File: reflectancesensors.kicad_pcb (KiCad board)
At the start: 2 copper layers, 71.5 x 47 mm, 22 parts, among them J1 Power, J2 Outputs, Q1 BPW40, Q2 BPW40, U1 TCRT5000L, U3 TCRT5000L

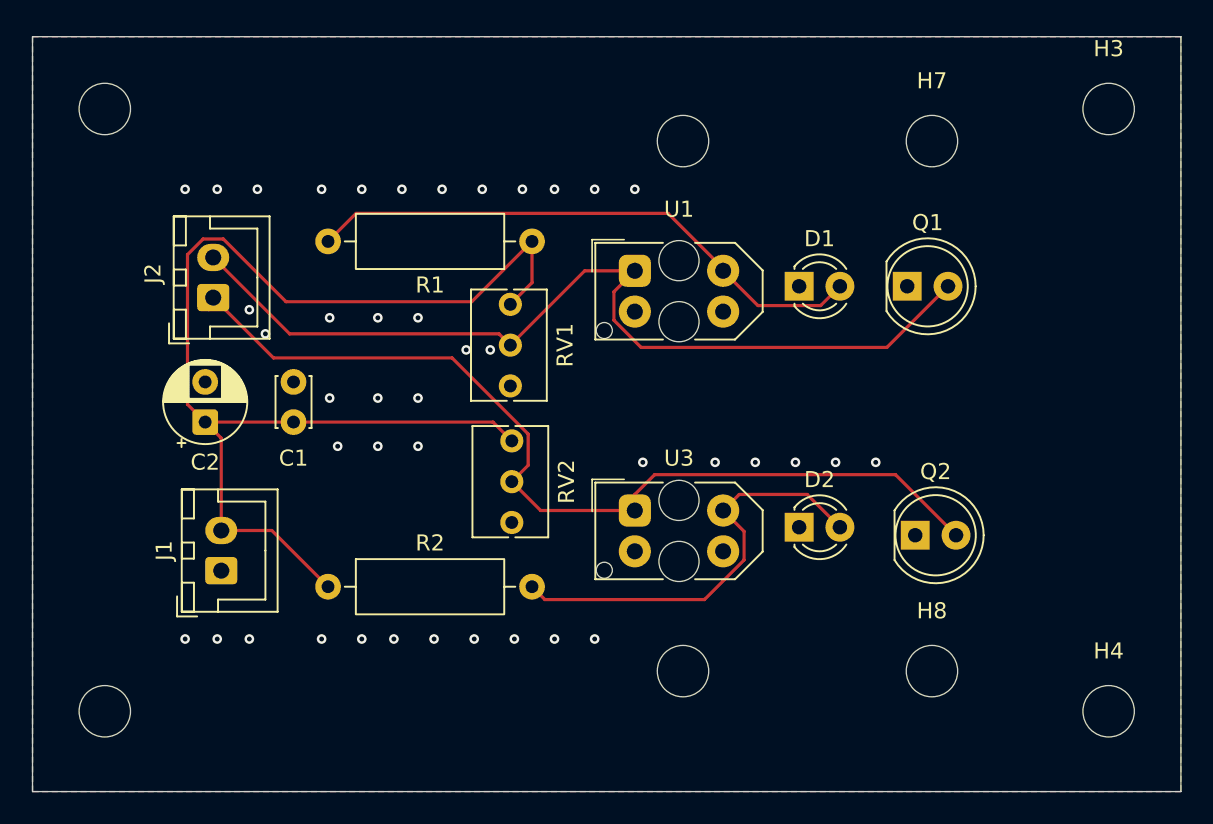
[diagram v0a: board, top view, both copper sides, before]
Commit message: small changes
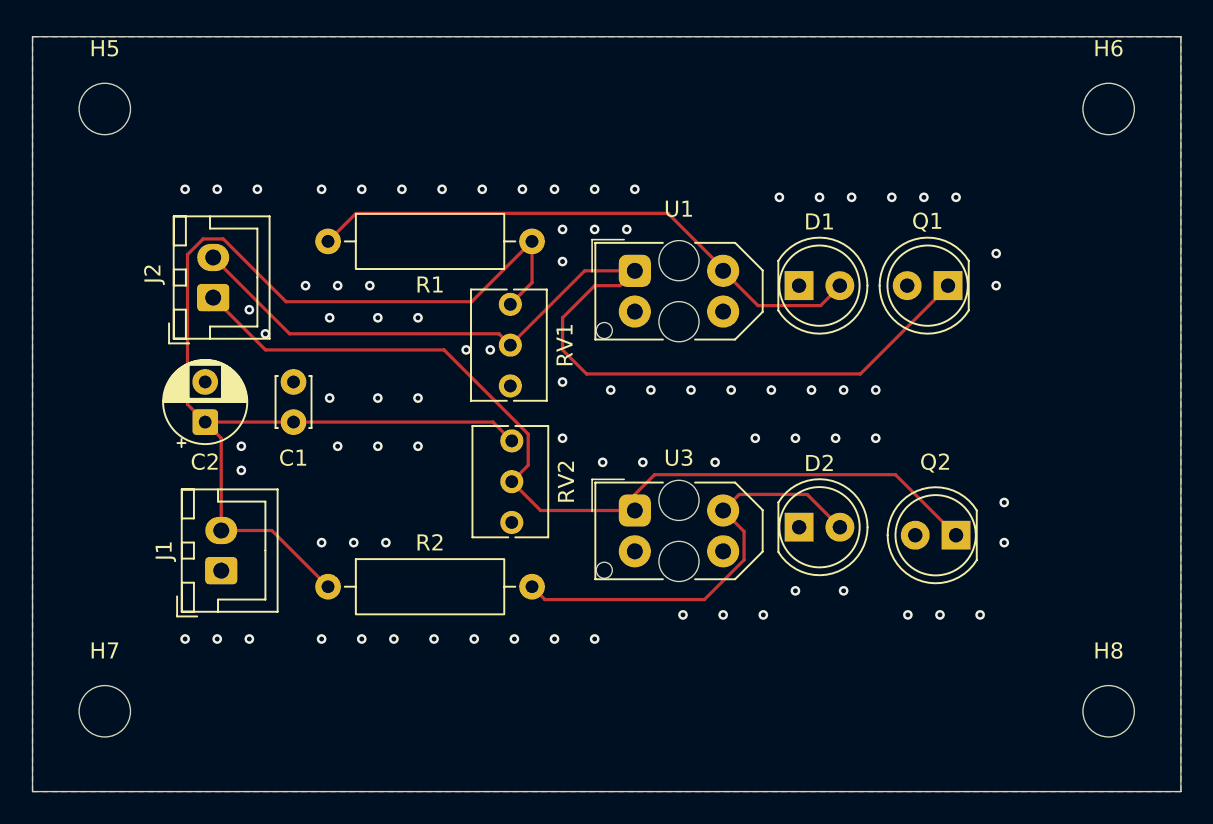
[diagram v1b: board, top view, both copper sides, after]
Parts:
- removed H1, H2, H3, H4: MountingHole, MountingHole:MountingHole_3.2mm_M3_DIN965
- D1, D2: footprint LED_THT:LED_D3.0mm_IRBlack -> LED_THT:LED_D5.0mm
- moved H7 62.5 mm to (82.5, 124.5)
- moved H6 43.9 mm to (145.0, 87.0)
- moved H5 36.1 mm to (82.5, 87.0)
- moved H8 11.3 mm to (145.0, 124.5)
- moved Q1 2.54 mm to (135.0, 98.0), turned to 180 degrees
- moved Q2 2.54 mm to (135.5, 113.5), turned to 180 degrees
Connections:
- Q1 pad 1: GND -> Net-(J2-Pin_2)
- Q1 pad 2: Net-(J2-Pin_2) -> GND
- Q2 pad 1: GND -> Net-(J2-Pin_1)
- Q2 pad 2: Net-(J2-Pin_1) -> GND
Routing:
- net Net-(J2-Pin_2): track 57.1 -> 65.0 mm
- net GND: vias 0 -> 83
- net (no net): vias 42 -> 0
